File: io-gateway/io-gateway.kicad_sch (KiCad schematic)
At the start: 8 parts, among them J1 1752201, J2 1752201, J3 1752201, J4 Screw_Terminal_01x09, J5 Screw_Terminal_01x09, J6 Screw_Terminal_01x09

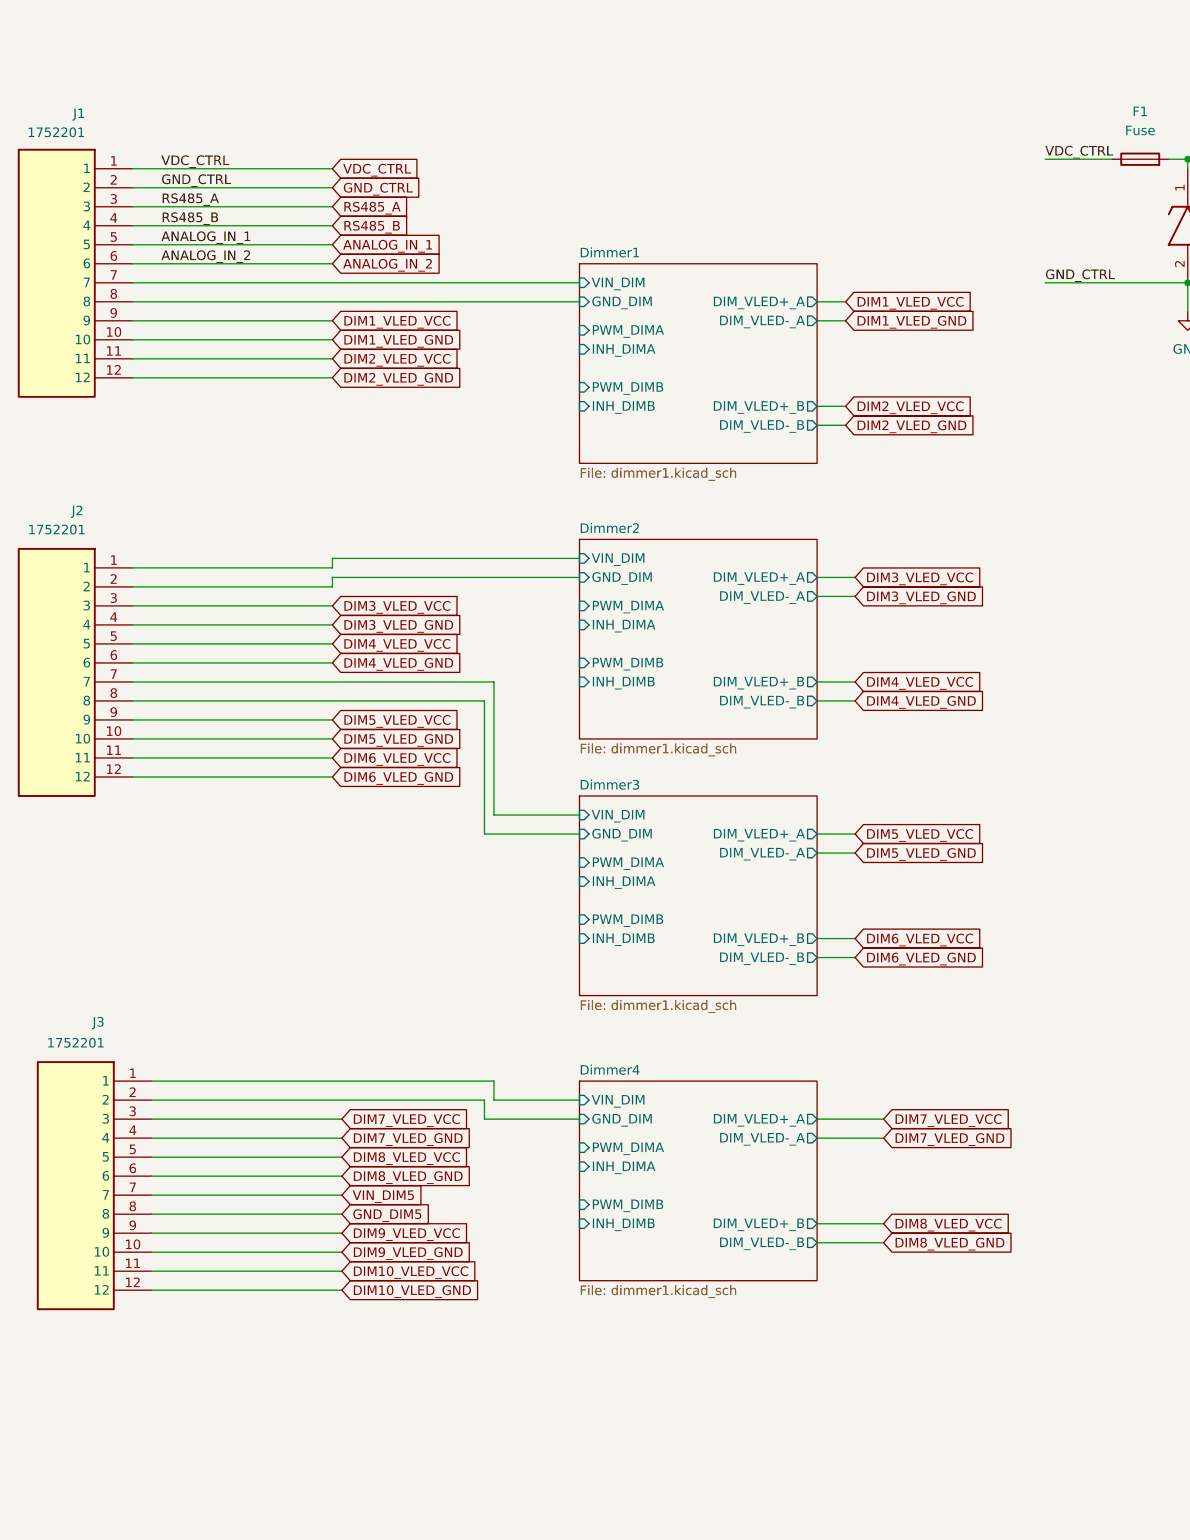
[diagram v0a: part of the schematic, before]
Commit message: upd
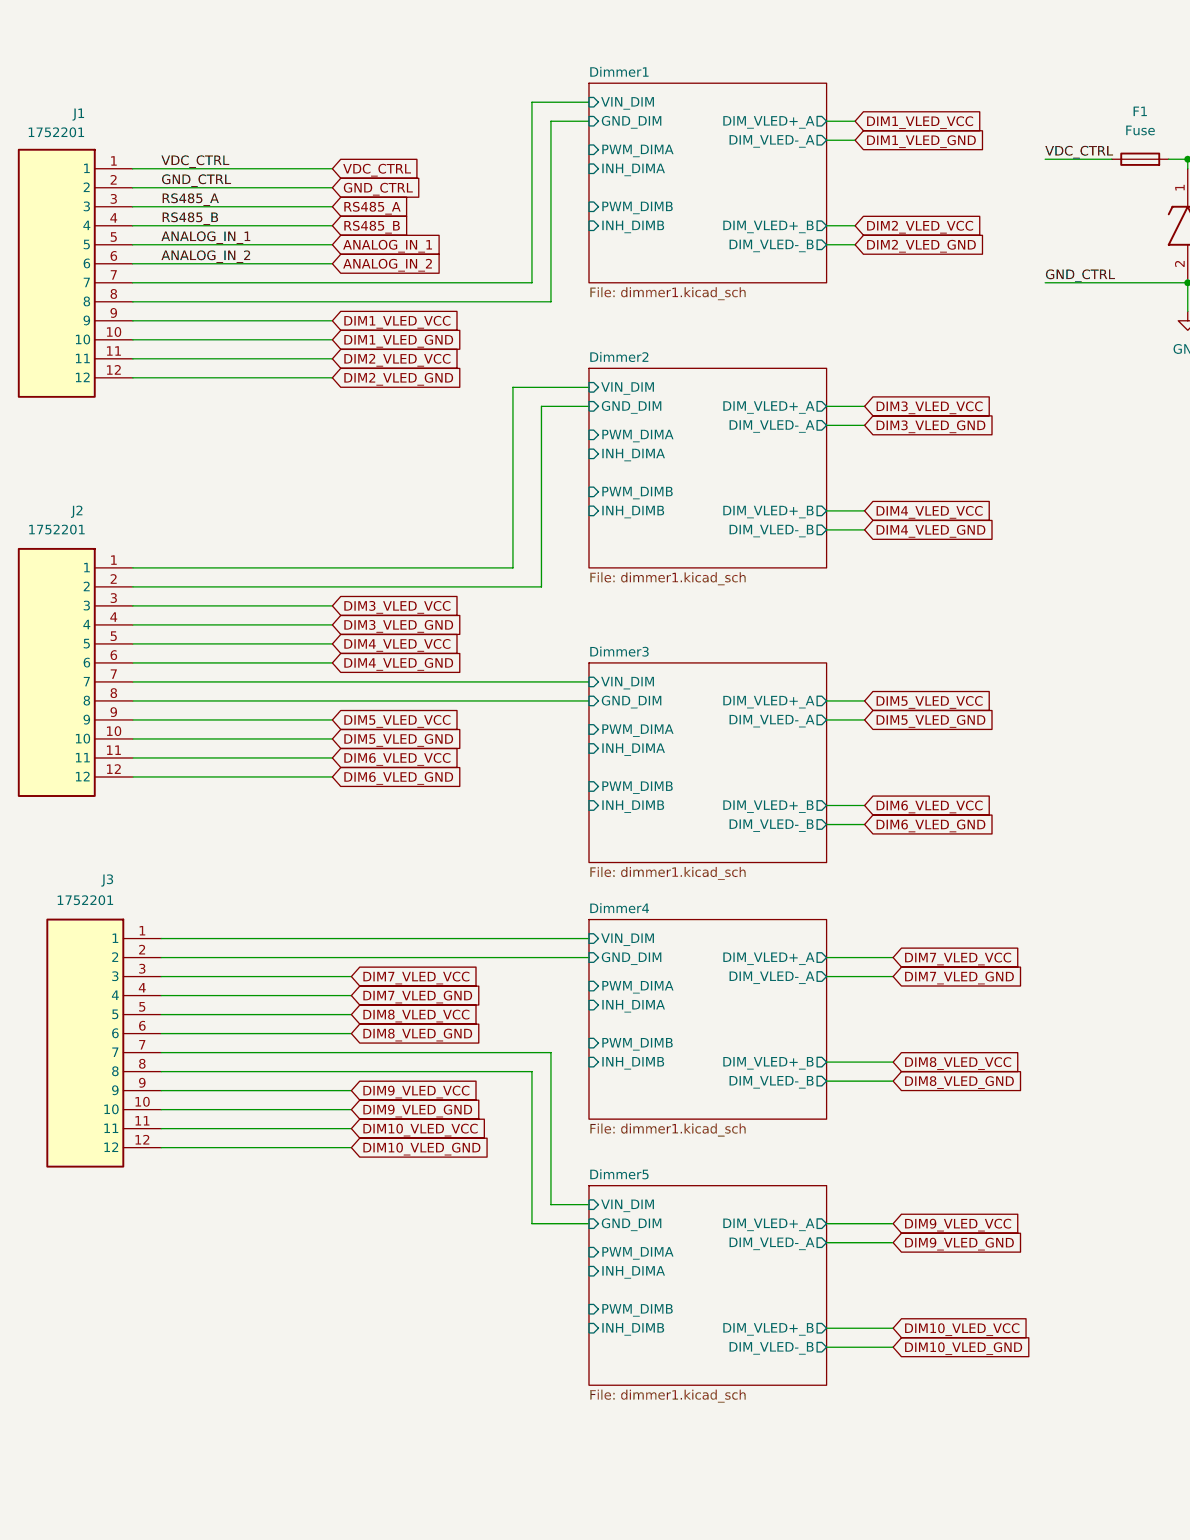
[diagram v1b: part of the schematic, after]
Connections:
- net GND_DIM5 renamed Dimmer5/GND_DIM
- net VIN_DIM5 renamed Dimmer5/VIN_DIM
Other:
- added sheet Dimmer5 (dimmer1.kicad_sch)
- moved on the sheet: J3
